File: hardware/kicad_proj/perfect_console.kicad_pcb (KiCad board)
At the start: 2 copper layers, 70 x 95 mm, 71 parts, among them J1 R_Out, J10 PWR_OUT_Pins, J11 GPIO_40-41, J12 USB_Out, J13 I2C, J14 ESP_UART, J15 GPIO10, J16 CH_UART, J17 CH_Flash, J18 Micro_SD_Card, J2 Jack_3.5, J3 L_Out, J4 USB, J5 TP4056_WO_Protect, J6 Bat, J7 PWR_Btn, J8 BTN_Pins, J9 PTT_Btn, Q1 NMOS, Q2 NMOS, Q3 NMOS, Q4 NMOS, Q5 NMOS, Q6 NMOS, SW1 Reset, SW2 Boot, U1 ESP32-S3-WROOM1, U2 Display, U3 PCM5102, U4 CH32V006E8R6, U5 PAM8403, U6 LoRa, U7 USBLC6-2SC6, U8 Mic, U9 DC-DC

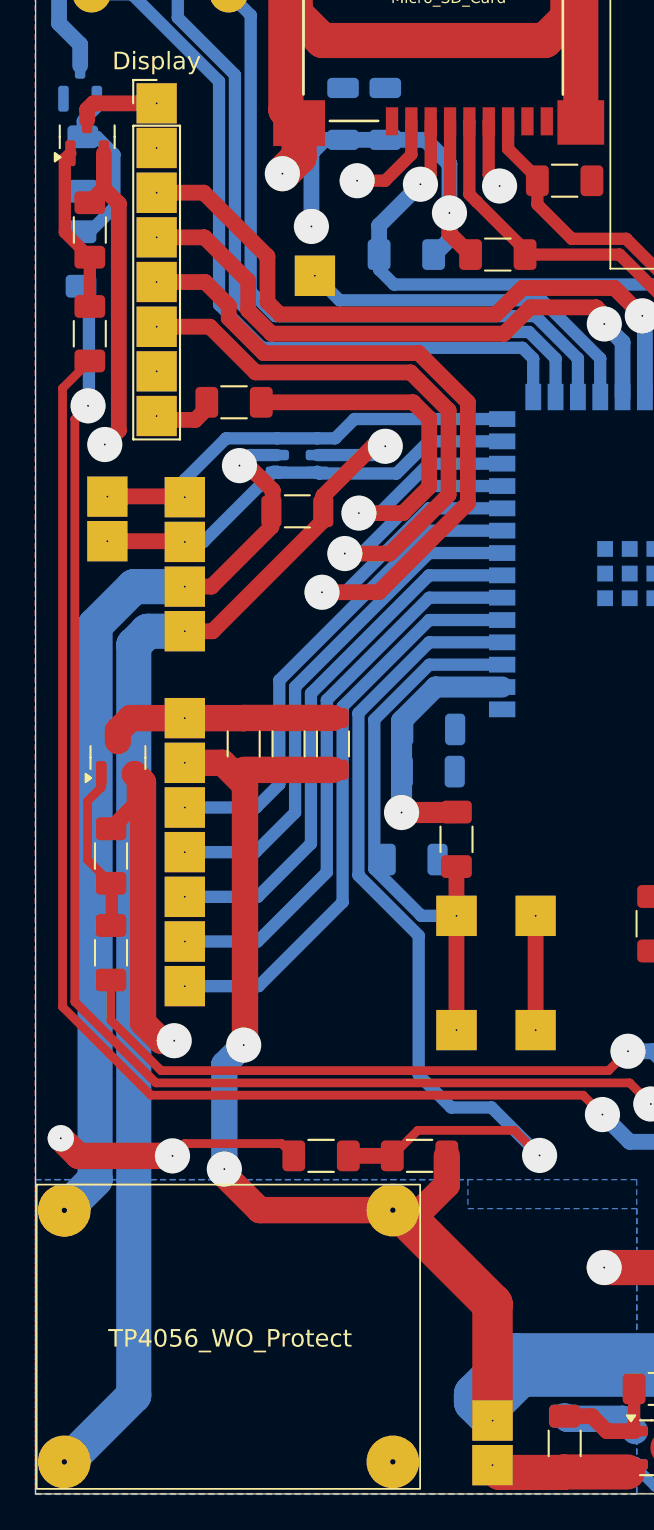
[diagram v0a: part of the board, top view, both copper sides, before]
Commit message: Виправлено схему
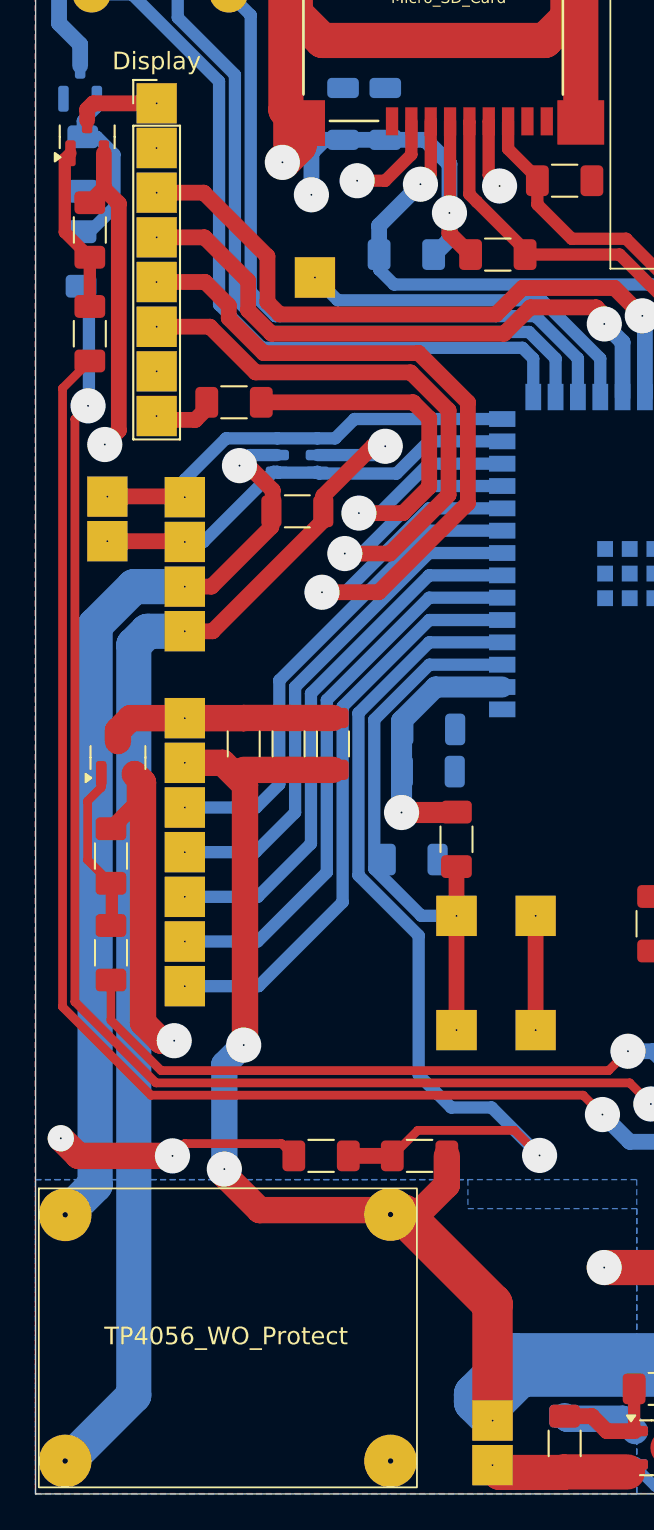
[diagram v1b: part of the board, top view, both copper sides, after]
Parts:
- moved J5 12.6 mm to (265.7, 227.9)
- moved J15 0.10 mm to (281.4, 176.1)
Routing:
- net +3V3: track 47.7 -> 45.9 mm
- net GND1: track 151.9 -> 151.3 mm
- net +4V2: track 244.4 -> 245.0 mm
